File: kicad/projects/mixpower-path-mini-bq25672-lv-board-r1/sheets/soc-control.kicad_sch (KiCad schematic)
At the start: 16 parts, among them Q7 BSS138PS, U6 STM32G071G8U6N, U8 TXS0102DQE

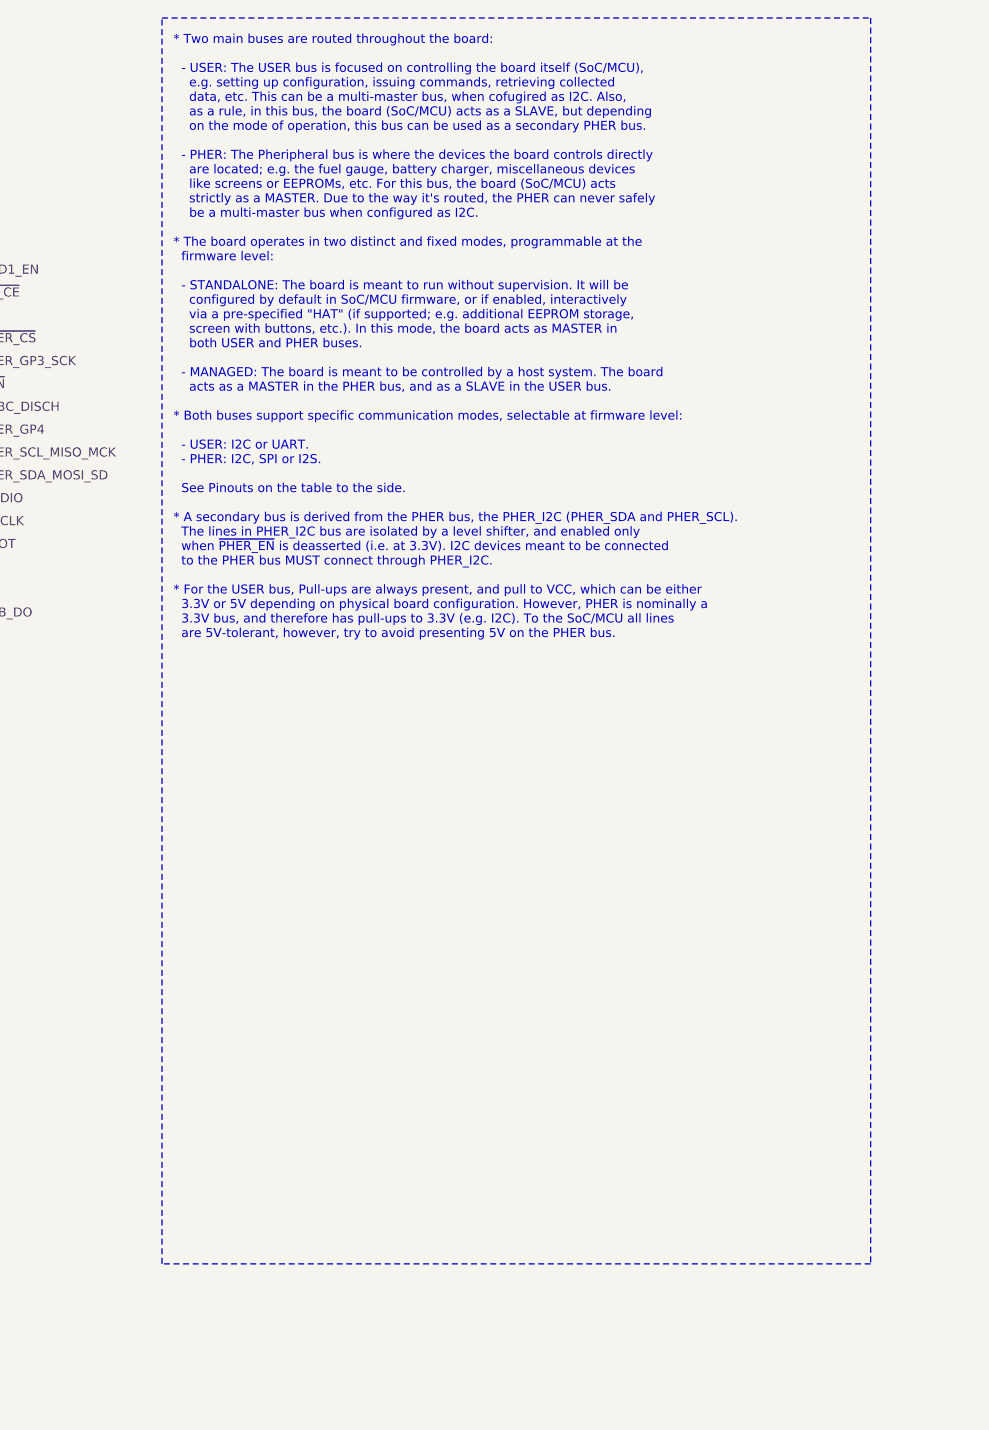
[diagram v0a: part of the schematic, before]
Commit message: feat: small changes in schematics, some PCB routing
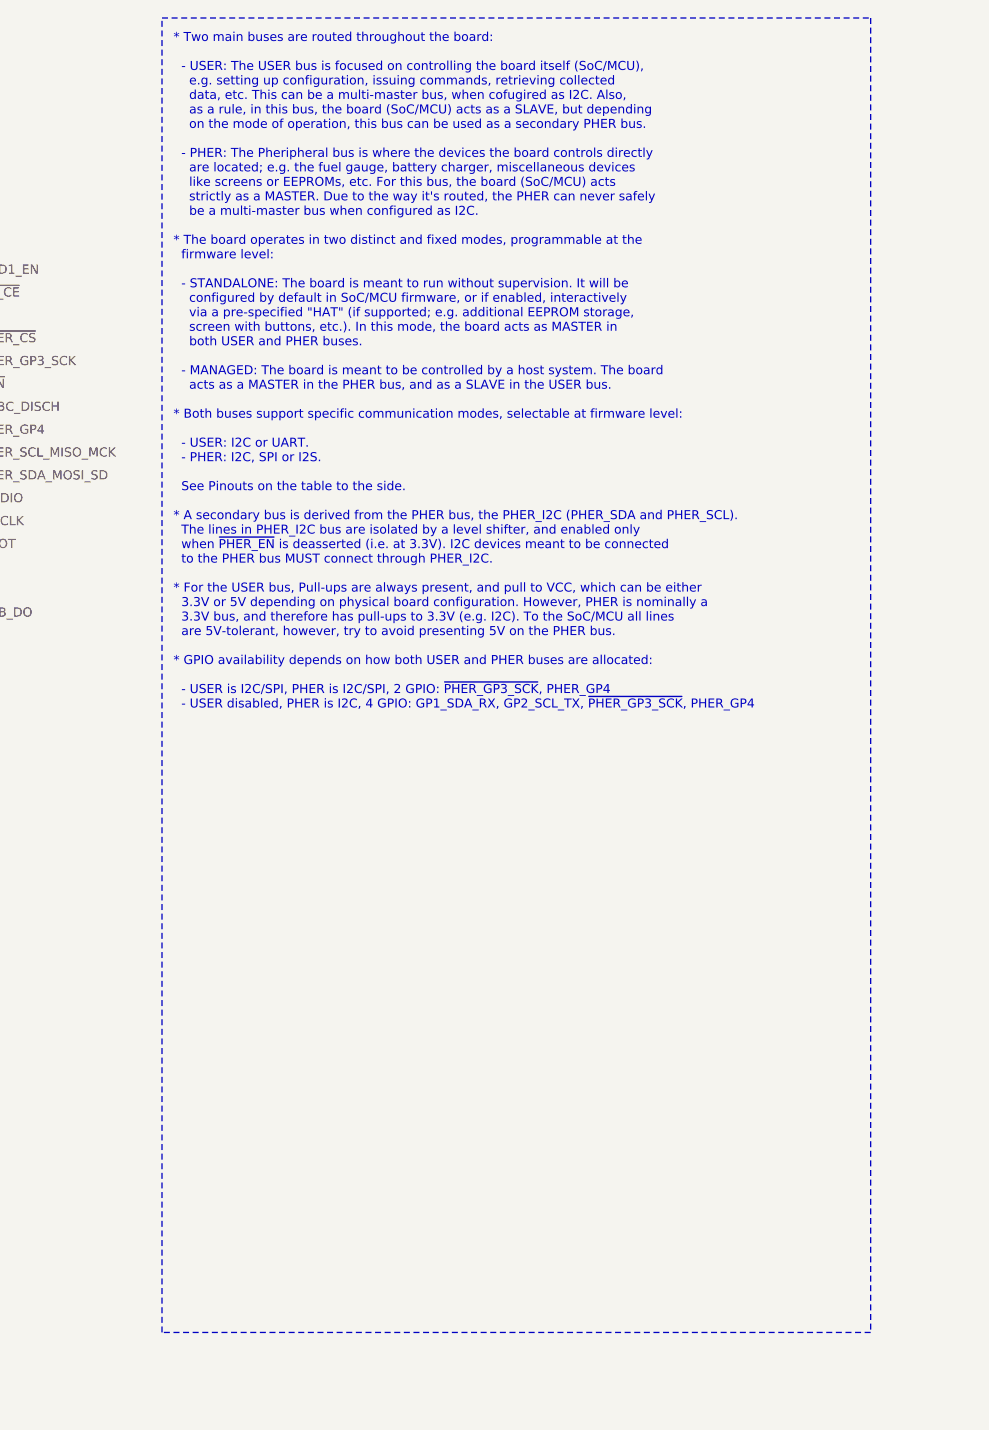
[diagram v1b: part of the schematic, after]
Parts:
- added unit 1 of D8
- added unit 3 of D8
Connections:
- net IRQB_TX: now also D8.6 (K2); no longer D8.6 (K2)
- net ~{IRQB}: now also D8.1 (A2); no longer D8.1 (A2)
- net ~{RGB_CS}: now also D8.4 (K3); no longer D8.4 (K3)
- net at D8.2 (A2), R41.2, U8.5 (OE): now also D8.3 (A3); no longer D8.3 (A3)

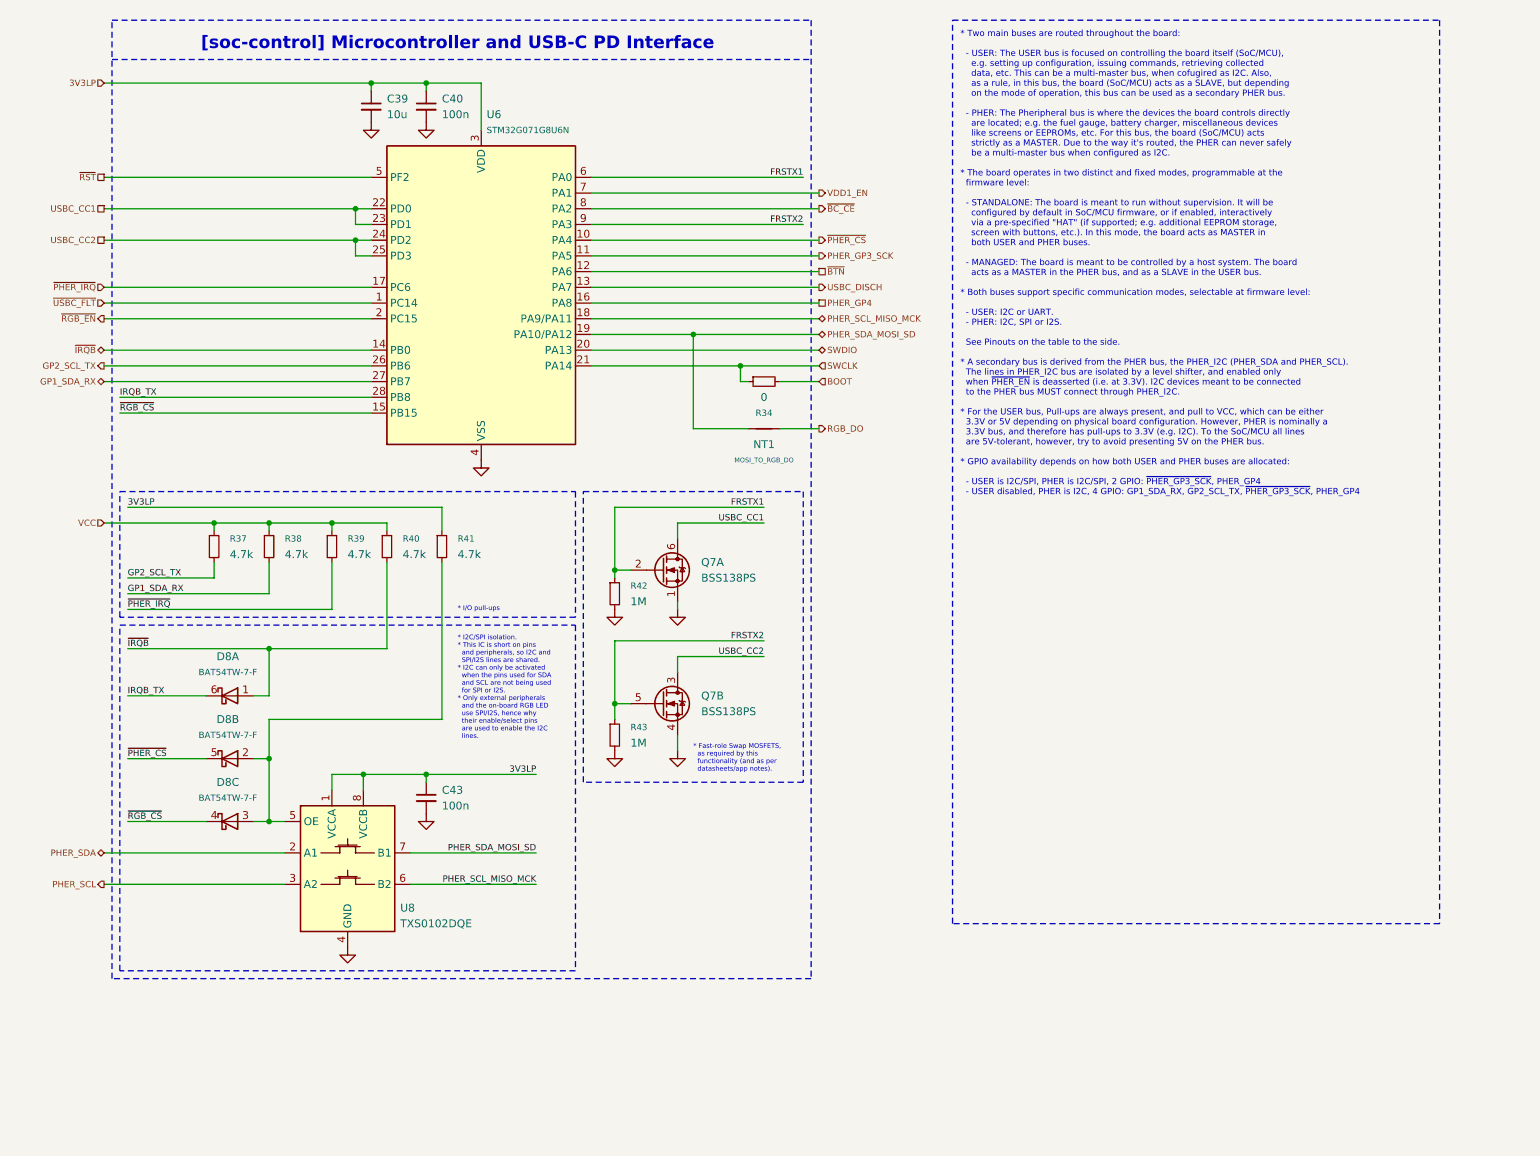
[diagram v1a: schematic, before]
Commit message: feat: failed PCB routing
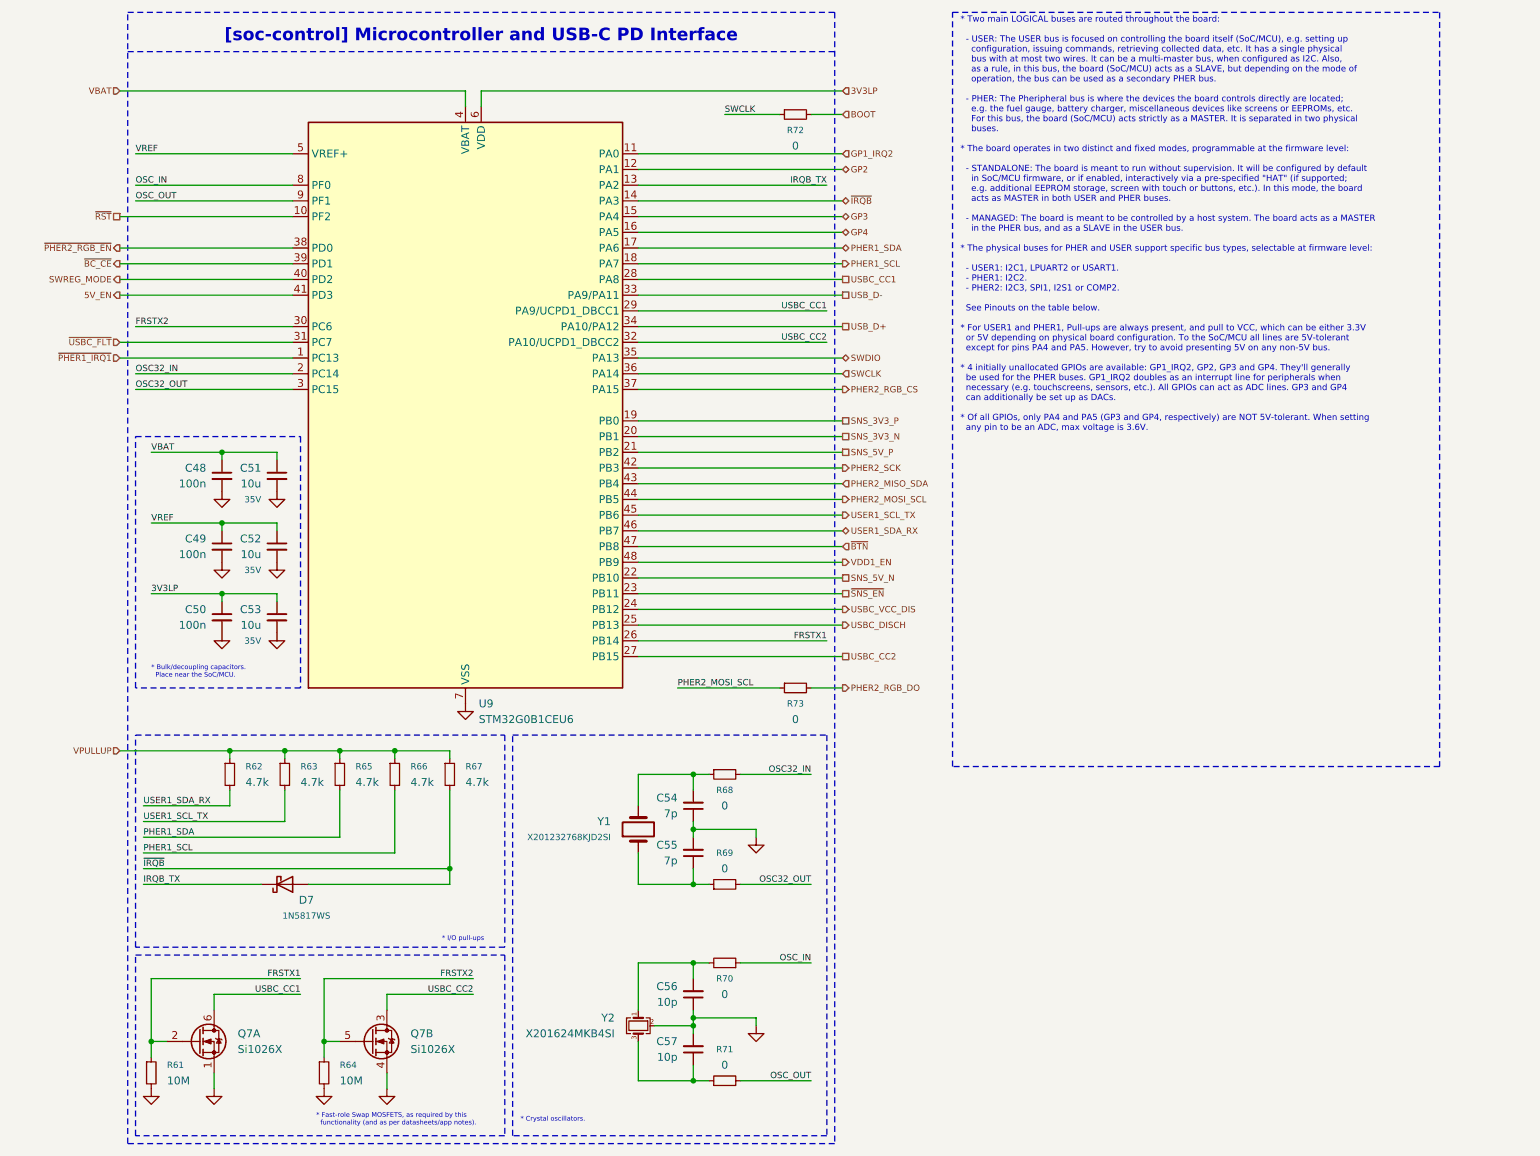
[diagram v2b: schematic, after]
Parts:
- removed C39: 10u, Capacitor_SMD:C_0603_1608Metric, symbol Device:C_Small
- removed C40, C43: 100n, Capacitor_SMD:C_0402_1005Metric, symbol Device:C_Small
- removed D8: BAT54TW-7-F, mixlib-generic-sot:SOT-363_SC-70-6, symbol mixlib-discrete-schottkydiode:BAT54TW
- removed NT1: MOSI_TO_RGB_DO, NetTie:NetTie-2_SMD_Pad0.5mm, symbol Device:NetTie_2
- removed Q7: BSS138PS, mixlib-generic-sot:SOT-363_SC-70-6, symbol mixlib-discrete-mosfet:BSS138PS
- removed R34: 0, Resistor_SMD:R_0402_1005Metric, symbol Device:R_Small
- removed R41: 4.7k, Resistor_SMD:R_0402_1005Metric, symbol Device:R_Small
- removed U6: STM32G071G8U6N, mixlib-vendor-st:QFN-28_4x4mm_P0.5mm, symbol mixlib-soc-stm32g0:STM32G071G8UxN
- removed U8: TXS0102DQE, Package_SON:X2SON-8_1.4x1mm_P0.35mm, symbol Logic_LevelTranslator:TXS0102DQE
- added C48, C49, C50: 100n, Capacitor_SMD:C_0402_1005Metric, symbol Device:C_Small
- added C51, C52, C53: 10u, Capacitor_SMD:C_0402_1005Metric, symbol Device:C_Small
- added C54, C55: 7p, Capacitor_SMD:C_0402_1005Metric, symbol Device:C_Small
- added C56, C57: 10p, Capacitor_SMD:C_0402_1005Metric, symbol Device:C_Small
- added D7: 1N5817WS, Diode_SMD:D_SOD-323, symbol Diode:1N5819WS
- added Q7: Si1026X, mixlib-generic-sot:SOT-563, symbol mixlib-discrete-mosfet:Si1026X
- added R67: 4.7k, Resistor_SMD:R_0402_1005Metric, symbol Device:R_Small
- added R68, R69, R70, R71, R72, R73: 0, Resistor_SMD:R_0402_1005Metric, symbol Device:R_Small
- added U9: STM32G0B1CEU6, Package_DFN_QFN:QFN-48-1EP_7x7mm_P0.5mm_EP5.6x5.6mm, symbol MCU_ST_STM32G0:STM32G0B1CEUx
- added Y1: X201232768KJD2SI, Crystal:Crystal_SMD_2012-2Pin_2.0x1.2mm, symbol Device:Crystal
- added Y2: X201624MKB4SI, Crystal:Crystal_SMD_2016-4Pin_2.0x1.6mm, symbol Device:Crystal_GND24_Small
- R61: renamed from R42; value 1M -> 10M
- R64: renamed from R43; value 1M -> 10M
- renumbered R37 to R62, R38 to R63, R39 to R65, R40 to R66
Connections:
- net 3V3LP: now also C50.1, C53.1, U9.6 (VDD)
- net BOOT: now also R72.2
- net FRSTX1: now also Q7.2 (G), U9.26 (PB14)
- net FRSTX2: now also Q7.5 (G), U9.30 (PC6)
- net GND: now also C48.2, C49.2, C50.2, C51.2, C52.2, C53.2, C54.1, C55.2, C56.1, C57.2, Q7.1 (S), Q7.4 (S), U9.49 (VSS), U9.7 (VSS), Y2.2 (G), Y2.4 (G)
- net IRQB_TX: now also D7.1 (K), U9.13 (PA2)
- net SWCLK: now also R72.1, U9.36 (PA14)
- net SWDIO: now also U9.35 (PA13)
- net USBC_CC1: now also Q7.6 (D), U9.28 (PA8), U9.29 (PA9/UCPD1_DBCC1)
- net USBC_CC2: now also Q7.3 (D), U9.27 (PB15), U9.32 (PA10/UCPD1_DBCC2)
- net USBC_DISCH: now also U9.25 (PB13)
- net VDD1_EN: now also U9.48 (PB9)
- net ~{BC_CE}: now also U9.39 (PD1)
- net ~{BTN}: now also U9.47 (PB8)
- net ~{IRQB}: now also D7.2 (A), R67.2, U9.14 (PA3); no longer R66.2
- net ~{RST}: now also U9.10 (PF2)
- net ~{USBC_FLT}: now also U9.31 (PC7)
- net GP1_SDA_RX renamed USER1_SCL_TX
- net USER1_SCL_TX: now also U9.45 (PB6)
- net GP2_SCL_TX renamed USER1_SDA_RX
- net USER1_SDA_RX: now also U9.46 (PB7)
- net VCC renamed VPULLUP
- net VPULLUP: now also R67.1
- net ~{PHER_IRQ} renamed PHER1_SDA
- net PHER1_SDA: now also U9.17 (PA6)
- new net: C56.2, R70.2, Y2.1
- new net: C57.1, R71.1, Y2.3
- new net: C55.1, R69.1, Y1.1
- new net: C54.2, R68.1, Y1.2
- new net 5V_EN: U9.41 (PD3)
- new net GP1_IRQ2: U9.11 (PA0)
- new net GP2: U9.12 (PA1)
- new net GP3: U9.15 (PA4)
- new net GP4: U9.16 (PA5)
- new net OSC32_IN: R68.2, U9.2 (PC14)
- new net OSC32_OUT: R69.2, U9.3 (PC15)
- new net OSC_IN: R70.1, U9.8 (PF0)
- new net OSC_OUT: R71.2, U9.9 (PF1)
- new net PHER1_SCL: R66.2, U9.18 (PA7)
- new net PHER2_MISO_SDA: U9.43 (PB4)
- new net PHER2_MOSI_SCL: R73.1, U9.44 (PB5)
- new net PHER2_RGB_CS: U9.37 (PA15)
- new net PHER2_RGB_DO: R73.2
- new net PHER2_SCK: U9.42 (PB3)
- new net SNS_3V3_N: U9.20 (PB1)
- new net SNS_3V3_P: U9.19 (PB0)
- new net SNS_5V_N: U9.22 (PB10)
- new net SNS_5V_P: U9.21 (PB2)
- new net SWREG_MODE: U9.40 (PD2)
- new net USBC_VCC_DIS: U9.24 (PB12)
- new net USB_D+: U9.34 (PA10/PA12)
- new net USB_D-: U9.33 (PA9/PA11)
- new net VBAT: C48.1, C51.1, U9.4 (VBAT)
- new net VREF: C49.1, C52.1, U9.5 (VREF+)
- new net ~{PHER1_IRQ1}: U9.1 (PC13)
- new net ~{PHER2_RGB_EN}: U9.38 (PD0)
- new net ~{SNS_EN}: U9.23 (PB11)
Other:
- note added: "* Bulk/decoupling capacitors. Place near the SoC/MCU."
- note added: "* Crystal oscillators."
- note added: "* Two main LOGICAL buses are routed throughout the board: - USER: The USER bus is focused on controlling the board itself (SoC/MCU), e.g. setting up configuration, issuing commands, retrieving collected data, etc. It has a single physical bus with at most two wires. It can be a multi-master bus, when configured as I2C. Also, as a rule, in this bus, the board (SoC/MCU) acts as a SLAVE, but dependi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"
- note removed: "* I2C/SPI isolation. * This IC is short on pins and peripherals, so I2C and SPI/I2S lines are shared. * I2C can only be activated when the pins used for SDA and SCL are not being used for SPI or I2S. * Only external peripherals and the on-board RGB LED use SPI/I2S, hence why their enable/select pins are used to enable the I2C lines."
- note removed: "* Two main buses are routed throughout the board: - USER: The USER bus is focused on controlling the board itself (SoC/MCU), e.g. setting up configuration, issuing commands, retrieving collected data, etc. This can be a multi-master bus, when cofugired as I2C. Also, as a rule, in this bus, the board (SoC/MCU) acts as a SLAVE, but depending on the mode of operation, this bus can be used as a secon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"
- moved on the sheet: R61, R62, R63, R64, R65, R66
